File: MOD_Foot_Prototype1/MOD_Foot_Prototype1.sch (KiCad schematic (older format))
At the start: 79 parts, among them CN1 CONN_PANNEL_2X2, CN2 CONN_PANNEL_2X2, J1 RJ45_CHAIN, J2 RJ45_CHAIN, P1 HEADER_5X1, P2 HEADER_5X2, Q1 MMBT3904, Q2 MMBT3904, U1 LPC111X_LQFP48, U2 MC7805, U3 NCP1117DT33G, U4 SN75176BDR, X1 10MHz

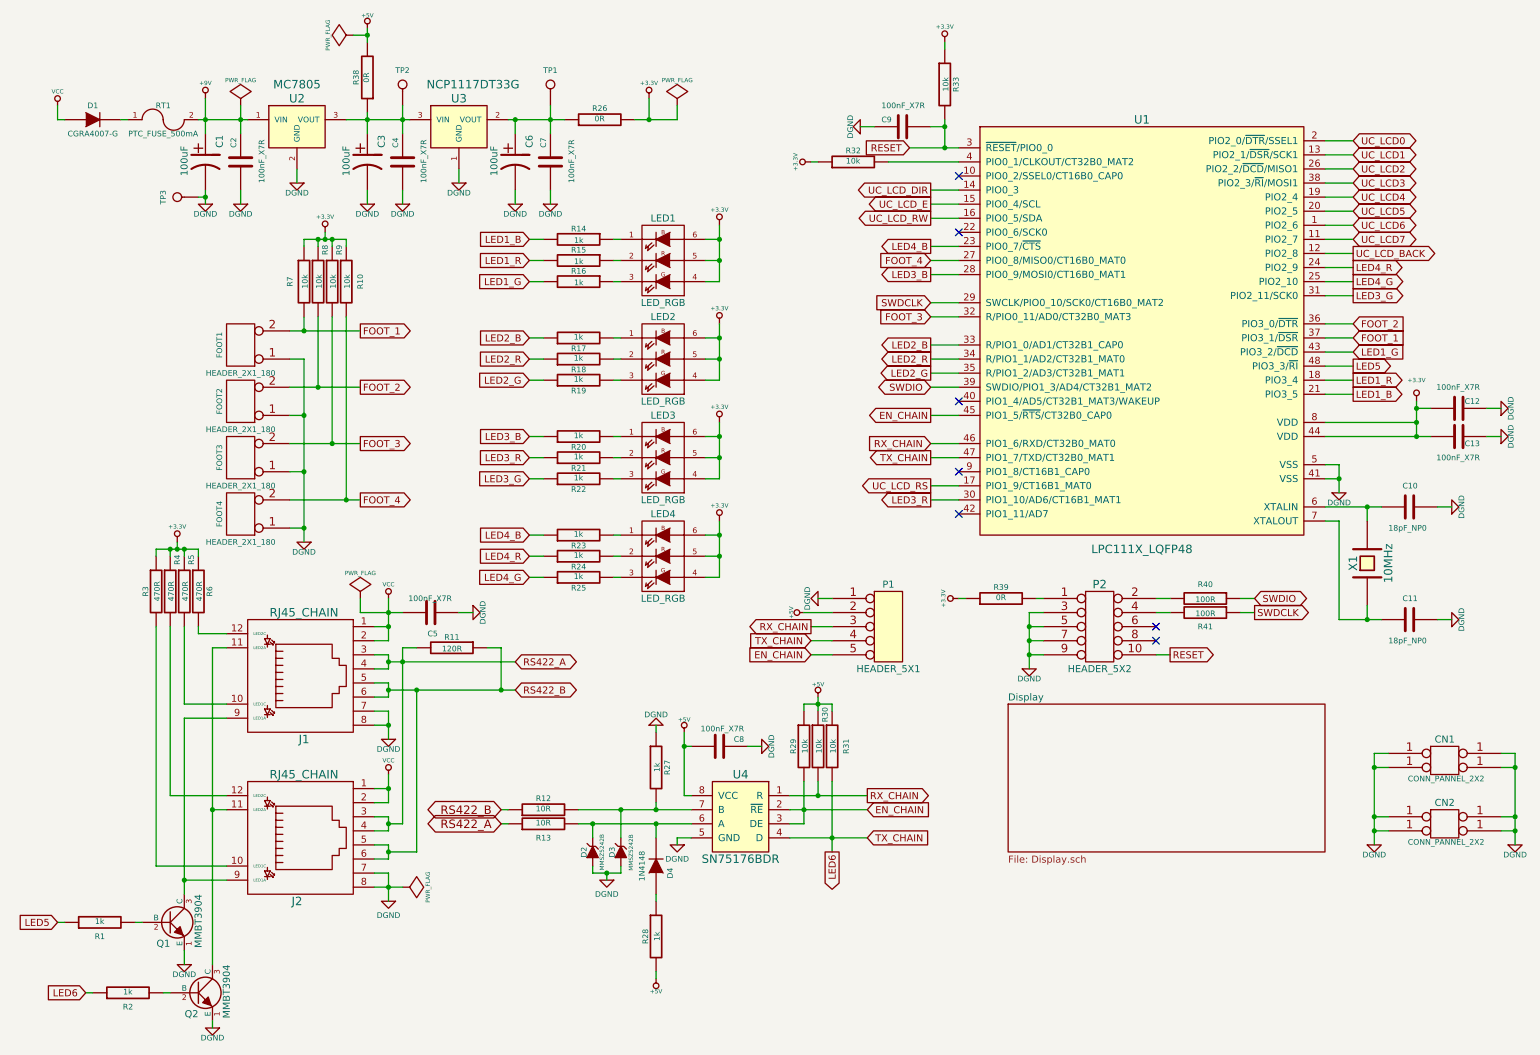
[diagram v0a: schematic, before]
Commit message: wip issue #11: protect the U4 IC when the board is being debugged - made the changes in the schematics
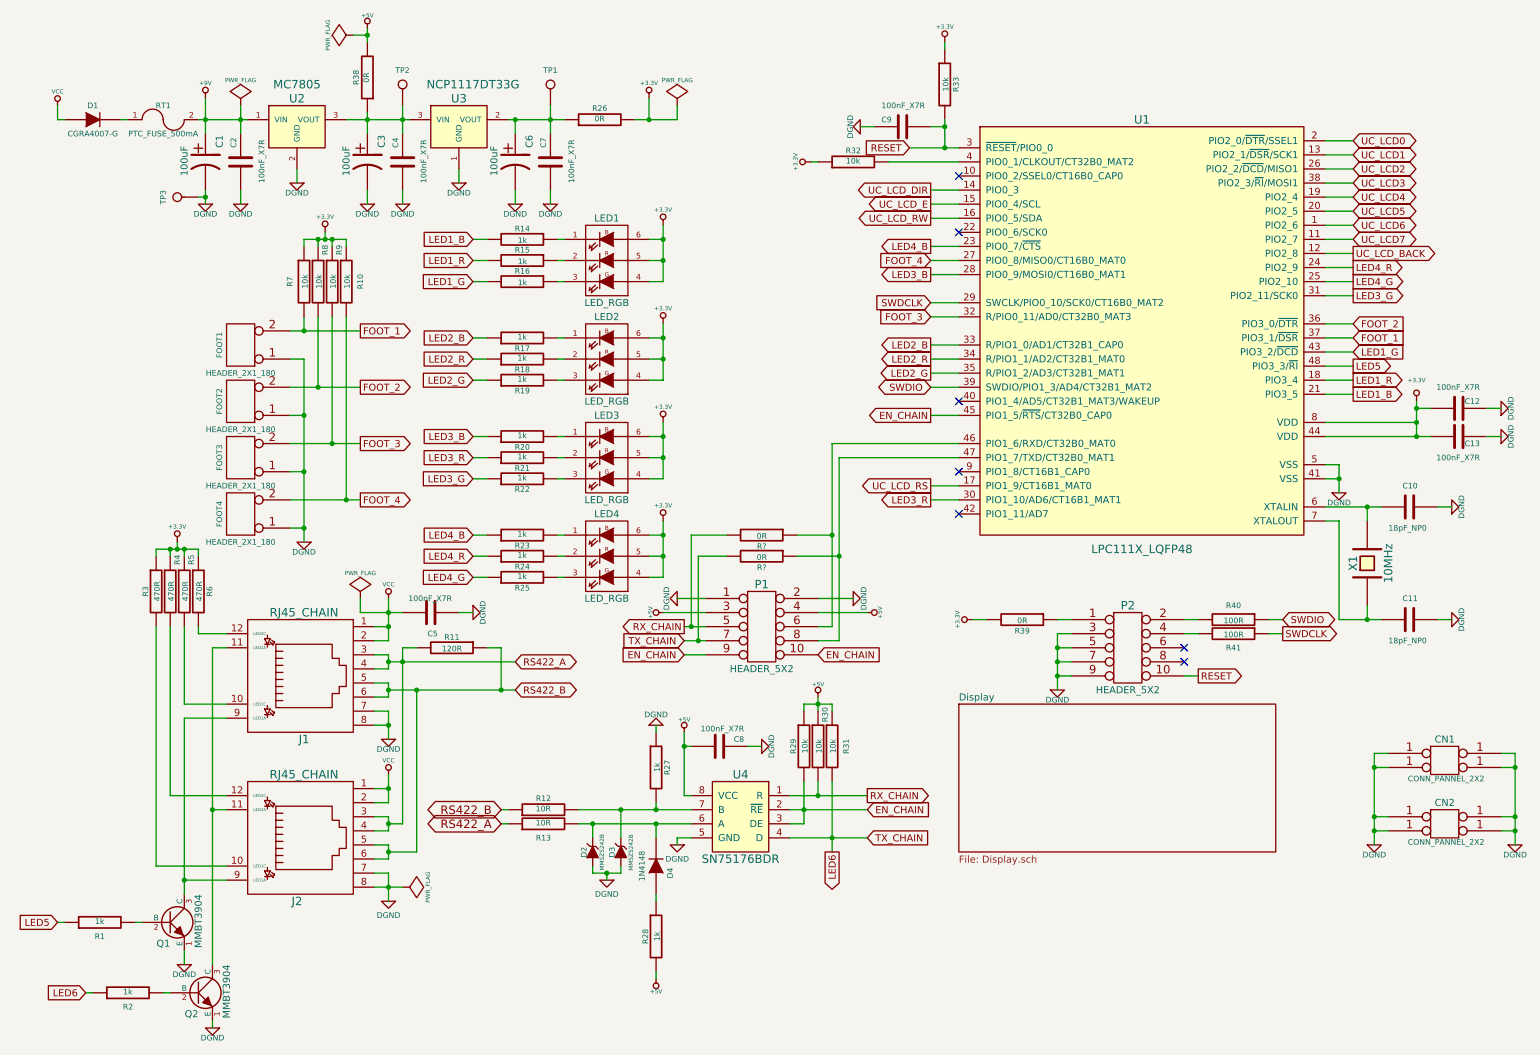
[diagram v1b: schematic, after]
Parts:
- removed P1: HEADER_5X1, MOD_Footprints_Lib:PIN_ARRAY_5x1, symbol CONN_5
- added P1: HEADER_5X2, MOD_Footprints_Lib:PIN_ARRAY_5x2, symbol CONN_5X2
- added R? (x2): 0R, MOD_Footprints_Lib:SM0805, symbol R
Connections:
- net +3.3V: now also R39.2; no longer R39.1
- net +5V: now also P1.3, P1.4
- net DGND: now also P1.1, P1.2
- net EN_CHAIN: now also P1.10, P1.9
- net LED6: now also P1.7, R?.2; no longer U1.47 (PIO1_7/TXD/CT32B0_MAT1)
- net RX_CHAIN: now also P1.5, R?.2; no longer U1.46 (PIO1_6/RXD/CT32B0_MAT0)
- net at P2.1: now also R39.1; no longer R39.2
- new net: P1.6, R?.1, U1.46 (PIO1_6/RXD/CT32B0_MAT0)
- new net: P1.8, R?.1, U1.47 (PIO1_7/TXD/CT32B0_MAT1)
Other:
- moved on the sheet: LED1, LED2, LED3, LED4, P2, R14, R15, R16, R17, R18, R19, R20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
